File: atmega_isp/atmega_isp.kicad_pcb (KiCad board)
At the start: 2 copper layers, 58.4 x 69.8 mm, 27 parts, among them J1 pwr, J2 analog, J3 ISP, J4 jmp, J5 jmp, J6 PD, J7 FTDI, J8 PB, J9 power, SW1 RST, U1 ATmega328P-AU, Y1 S3B20

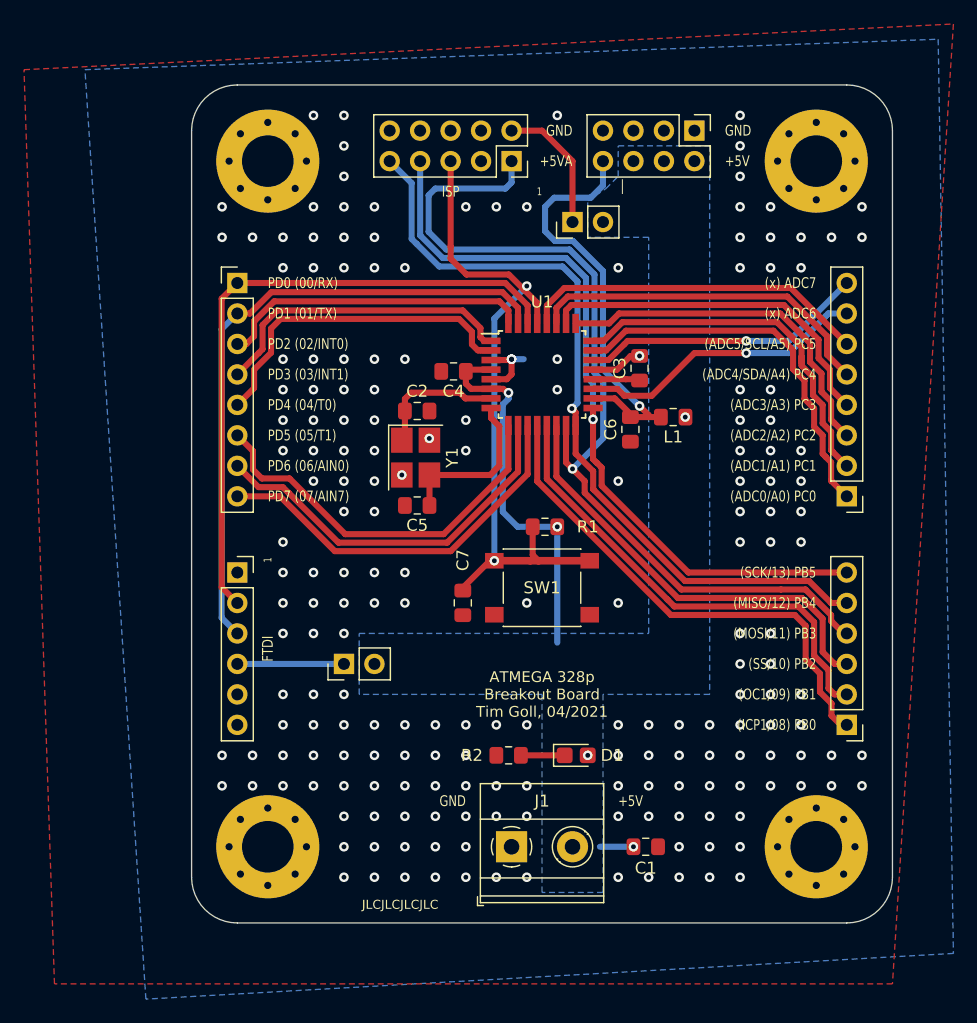
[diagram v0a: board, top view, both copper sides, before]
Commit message: kicad 6 update
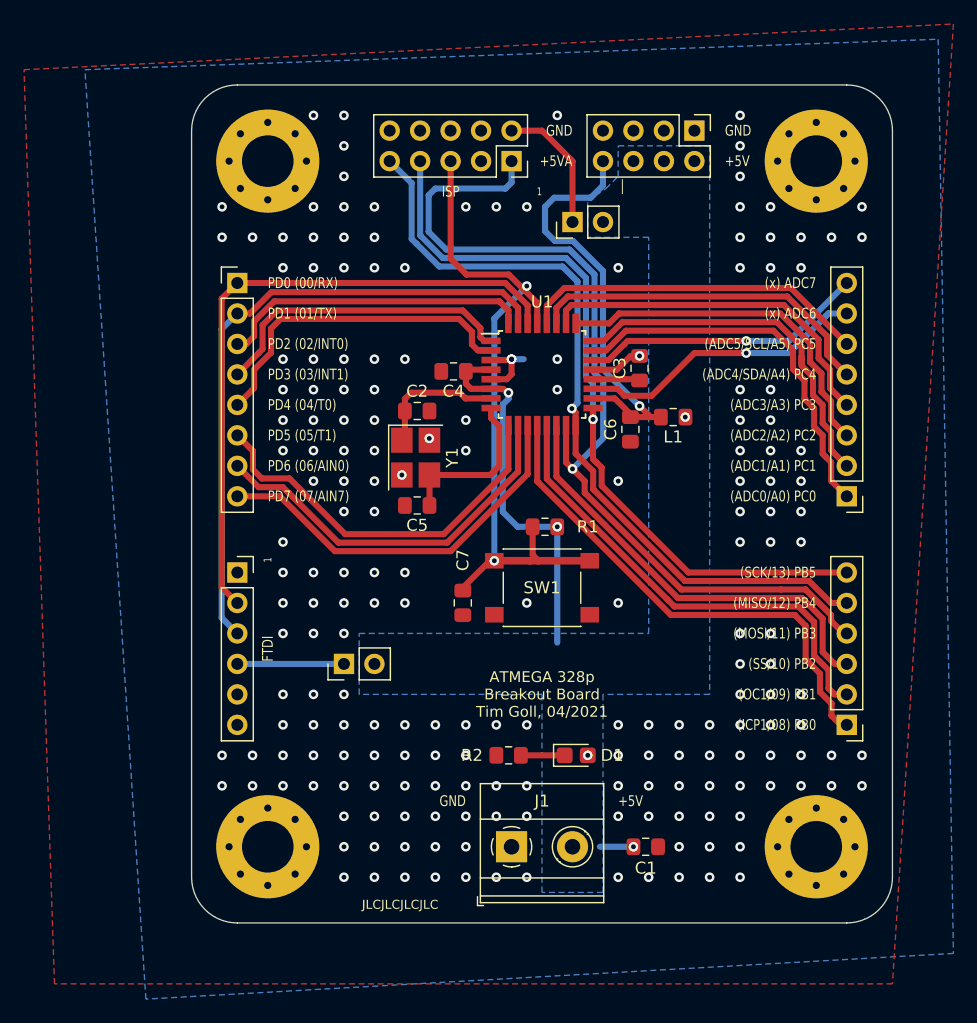
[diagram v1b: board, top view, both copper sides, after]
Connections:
- net ~RST renamed ~{RST}
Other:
- net class Default removed
